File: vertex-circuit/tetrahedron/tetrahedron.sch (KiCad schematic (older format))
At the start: 9 parts, among them J1 DIP-BLACK-MALE-HEADER-VERT_4P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, J2 DIP-BLACK-MALE-HEADER-VERT_4P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, J3 DIP-BLACK-MALE-HEADER-VERT_4P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, J4 DIP-BLACK-MALE-HEADER-VERT_4P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, J5 JACK-DC-005, J6 DIP-BLACK-MALE-HEADER-VERT_4P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, J7 DIP-BLACK-MALE-HEADER-VERT_4P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, J8 DIP-BLACK-MALE-HEADER-VERT_4P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

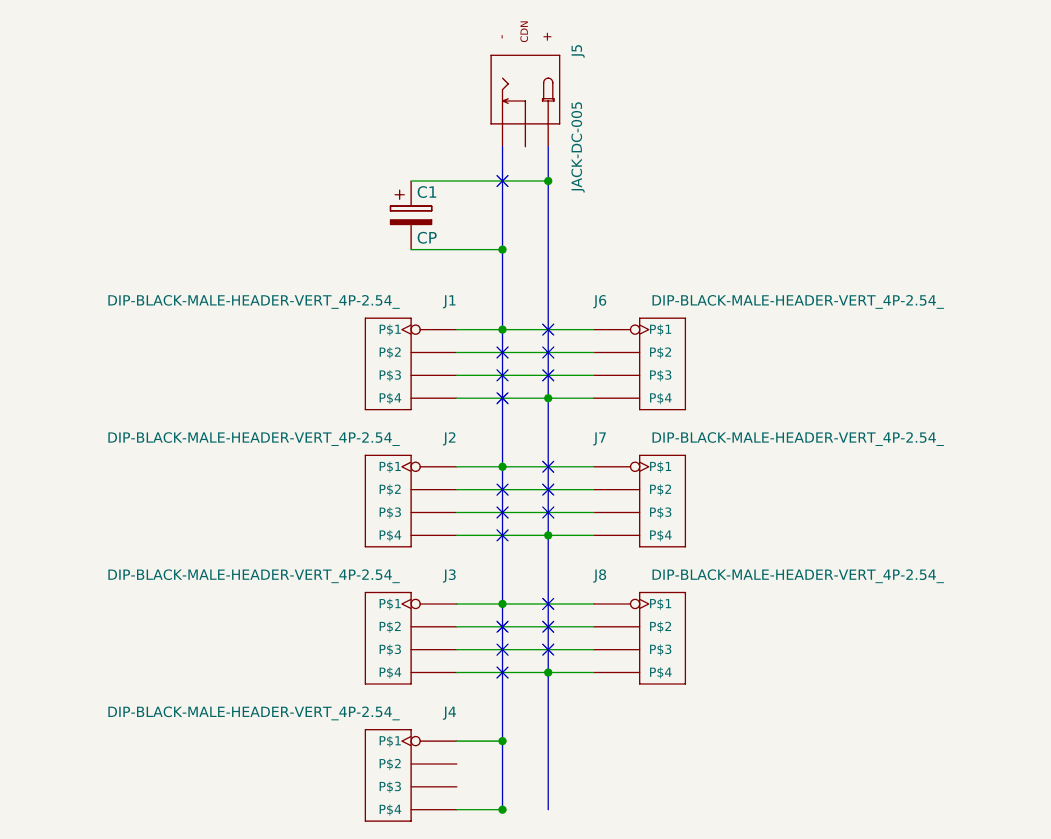
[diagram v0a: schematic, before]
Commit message: save circuits
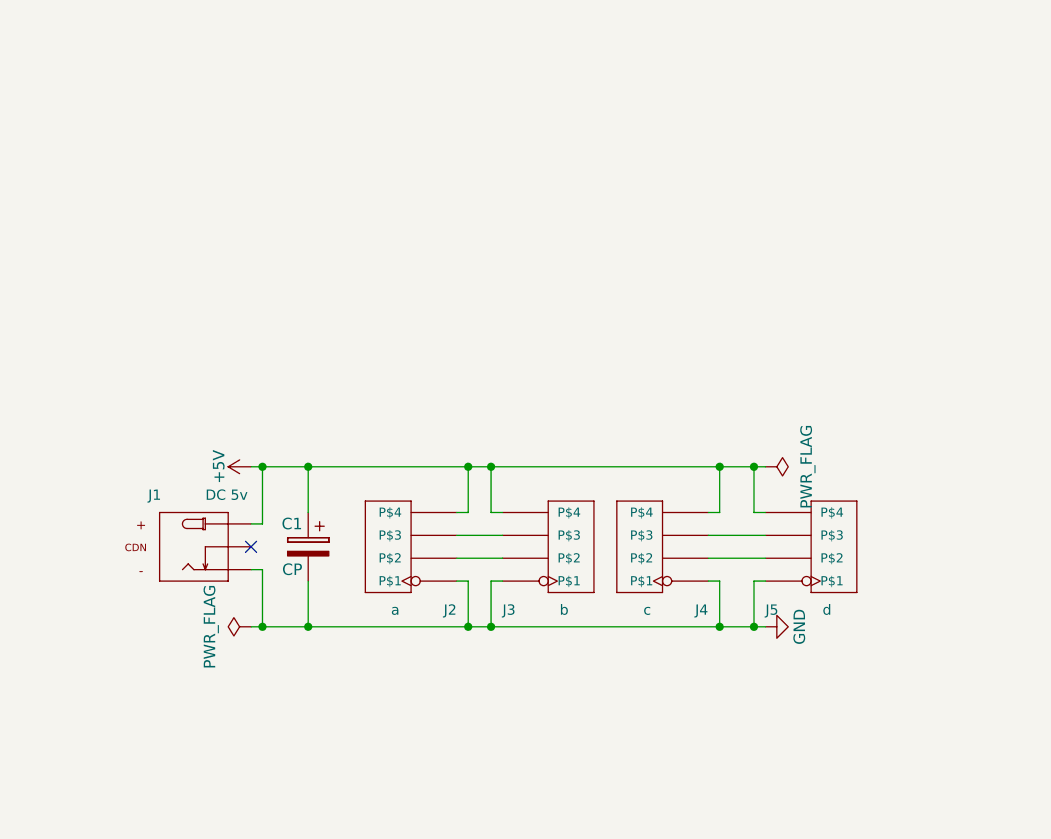
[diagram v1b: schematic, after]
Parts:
- removed J2, J3, J7, J8: DIP-BLACK-MALE-HEADER-VERT_4P-2.54_, SeeedOPL-Connector-2016:H4-2.54, symbol DIP-BLACK-MALE-HEADER-VERT_4P-2.54_
- added J5: d, SeeedOPL-Connector-2016:H4-2.54, symbol DIP-BLACK-MALE-HEADER-VERT_4P-2.54_
- J1: renamed from J5; value JACK-DC-005 -> DC 5v
- J2: renamed from J6; value DIP-BLACK-MALE-HEADER-VERT_4P-2.54_ -> a
- J3: renamed from J1; value DIP-BLACK-MALE-HEADER-VERT_4P-2.54_ -> b
- J4: value DIP-BLACK-MALE-HEADER-VERT_4P-2.54_ -> c
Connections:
- net GND: now reaches J2.1 (P$1), J3.1 (P$1)
- net GND: now also C1.2, J1.-1 (-), J4.1 (P$1), J5.1 (P$1)
- net +5V: now reaches J2.4 (P$4), J3.4 (P$4)
- net +5V: now also C1.1, J1.+, J4.4 (P$4), J5.4 (P$4)
- net at J4.2 (P$2): now also J5.2 (P$2)
- net at J4.3 (P$3): now also J5.3 (P$3)
- no-connect marks 19 -> 1
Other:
- moved on the sheet: C1, J1, J2, J3, J4
